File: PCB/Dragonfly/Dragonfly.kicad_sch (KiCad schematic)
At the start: 37 parts, among them J1 Conn_01x04_Pin, J2 Micro_SD_Card, SW1 SW_SPST, SW2 SW_SPST, U1 STM32F405RGTx, U2 ICM-20602, X1 TSX-3225

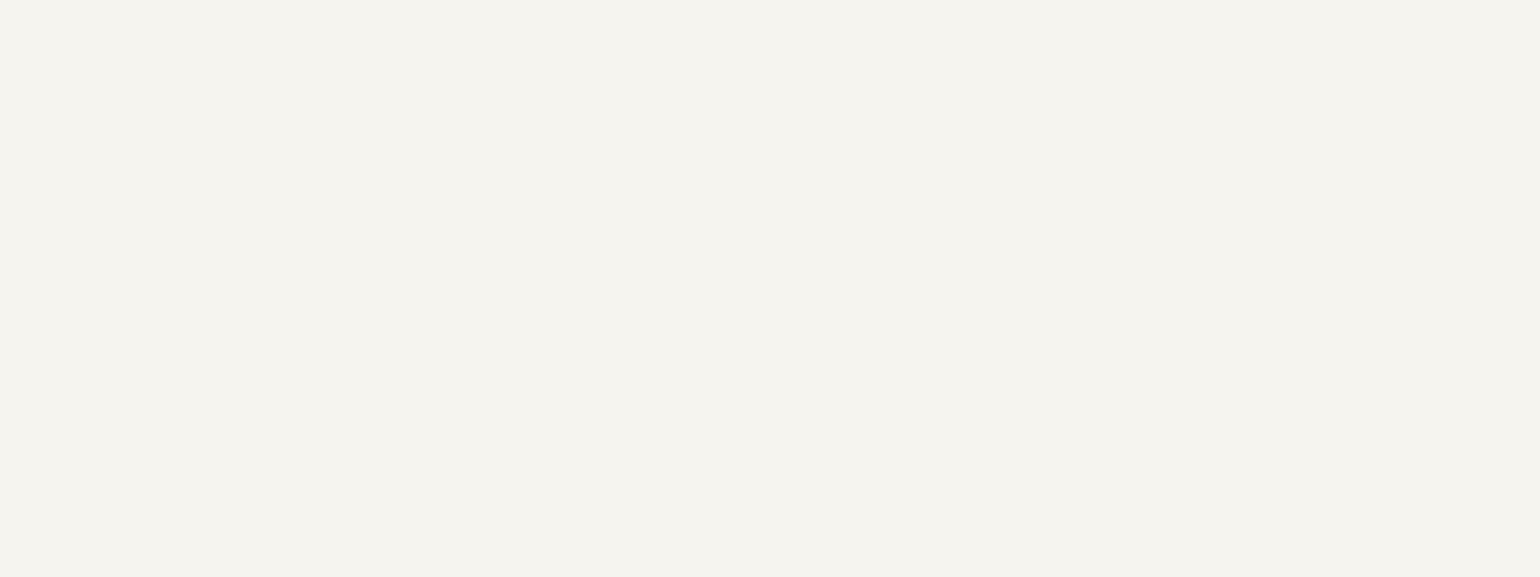
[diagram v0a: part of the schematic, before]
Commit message: wow
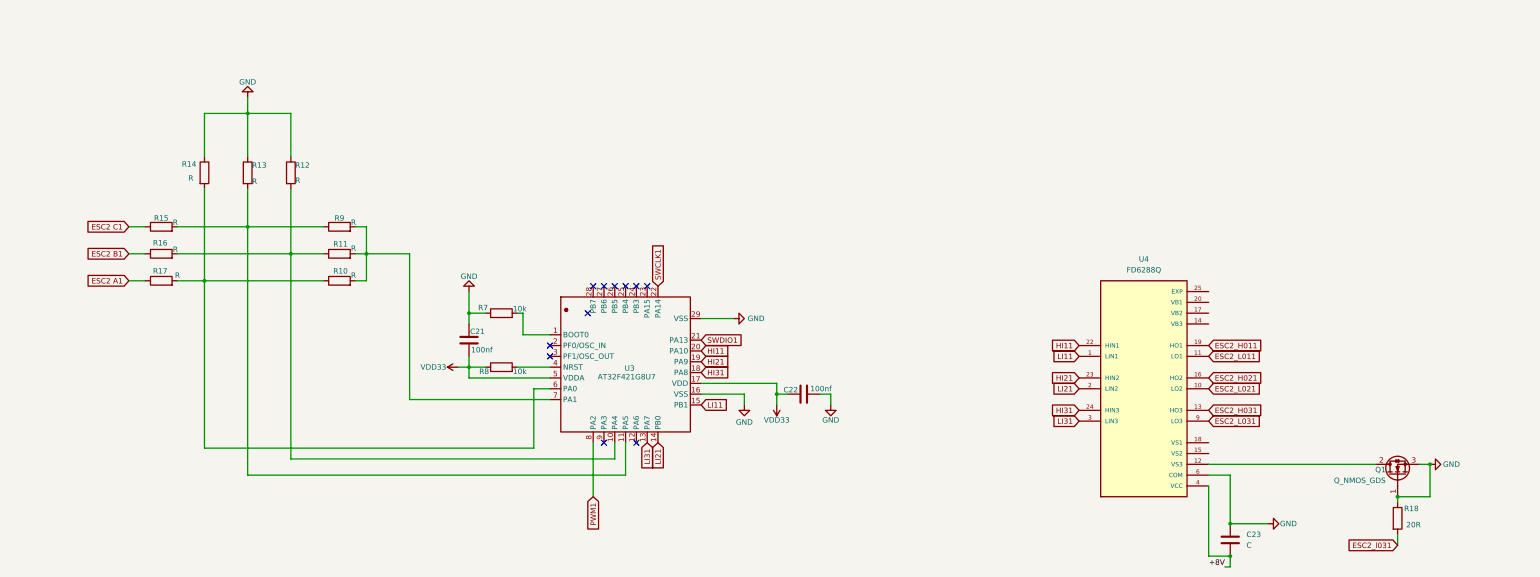
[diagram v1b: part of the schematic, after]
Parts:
- added C21, C22: 100nf, symbol Device:C
- added C23: C, symbol Device:C
- added Q1: Q_NMOS_GDS, symbol Transistor_FET:Q_NMOS_GDS
- added R10, R11, R12, R13, R14, R15, R16, R17, R9: R, symbol Device:R
- added R18: 20R, symbol Device:R
- added R7, R8: 10k, symbol Device:R
- added U3: AT32F421G8U7, AT32F421G8U7:AT32F421G8U7, symbol AT32F421G8U7:AT32F421G8U7
- added U4: FD6288Q, QFN50P400X400X90-25N, symbol FD6288Q:FD6288Q
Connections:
- net GND: now also C21.1, C22.2, C23.1, Q1.1 (G), Q1.3 (S), R12.1, R13.1, R14.1, R18.1, R7.1, U3.16 (VSS), U3.29 (VSS), U4.6 (COM)
- net VDD33: now also C21.2, C22.1, R8.1, U3.17 (VDD), U3.5 (VDDA)
- new net: R11.1, R12.2, R16.2, U3.10 (PA4)
- new net: R10.2, R11.2, R9.2, U3.7 (PA1)
- new net: R13.2, R15.2, R9.1, U3.11 (PA5)
- new net: R10.1, R14.2, R17.2, U3.6 (PA0)
- new net: Q1.2 (D), U4.12 (VS3)
- new net: R7.2, U3.1 (BOOT0)
- new net: R8.2, U3.4 (NRST)
- new net +8V: C23.2, U4.4 (VCC)
- new net ESC2 A1: R17.1
- new net ESC2 B1: R16.1
- new net ESC2 C1: R15.1
- new net ESC2_H011: U4.19 (HO1)
- new net ESC2_H021: U4.16 (HO2)
- new net ESC2_H031: U4.13 (HO3)
- new net ESC2_L011: U4.11 (LO1)
- new net ESC2_L021: U4.10 (LO2)
- new net ESC2_L031: U4.9 (LO3)
- new net ESC2_l031: R18.2
- new net HI11: U3.20 (PA10), U4.22 (HIN1)
- new net HI21: U3.19 (PA9), U4.23 (HIN2)
- new net HI31: U3.18 (PA8), U4.24 (HIN3)
- new net LI11: U3.15 (PB1), U4.1 (LIN1)
- new net LI21: U3.14 (PB0), U4.2 (LIN2)
- new net LI31: U3.13 (PA7), U4.3 (LIN3)
- new net PWM1: U3.8 (PA2)
- new net SWCLK1: U3.22 (PA14)
- new net SWDIO1: U3.21 (PA13)
- no-connect marks 0 -> 11
